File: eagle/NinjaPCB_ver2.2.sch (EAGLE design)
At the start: 70 parts, among them IC1 ANALOGSW_AD_SOT23-6, IC2 NAU7802, Q1 IRLB3813PBF, Q2 CJ2302, Q3 CJ2302, Q4 S9013, Q5 S9013, Q6 S9013

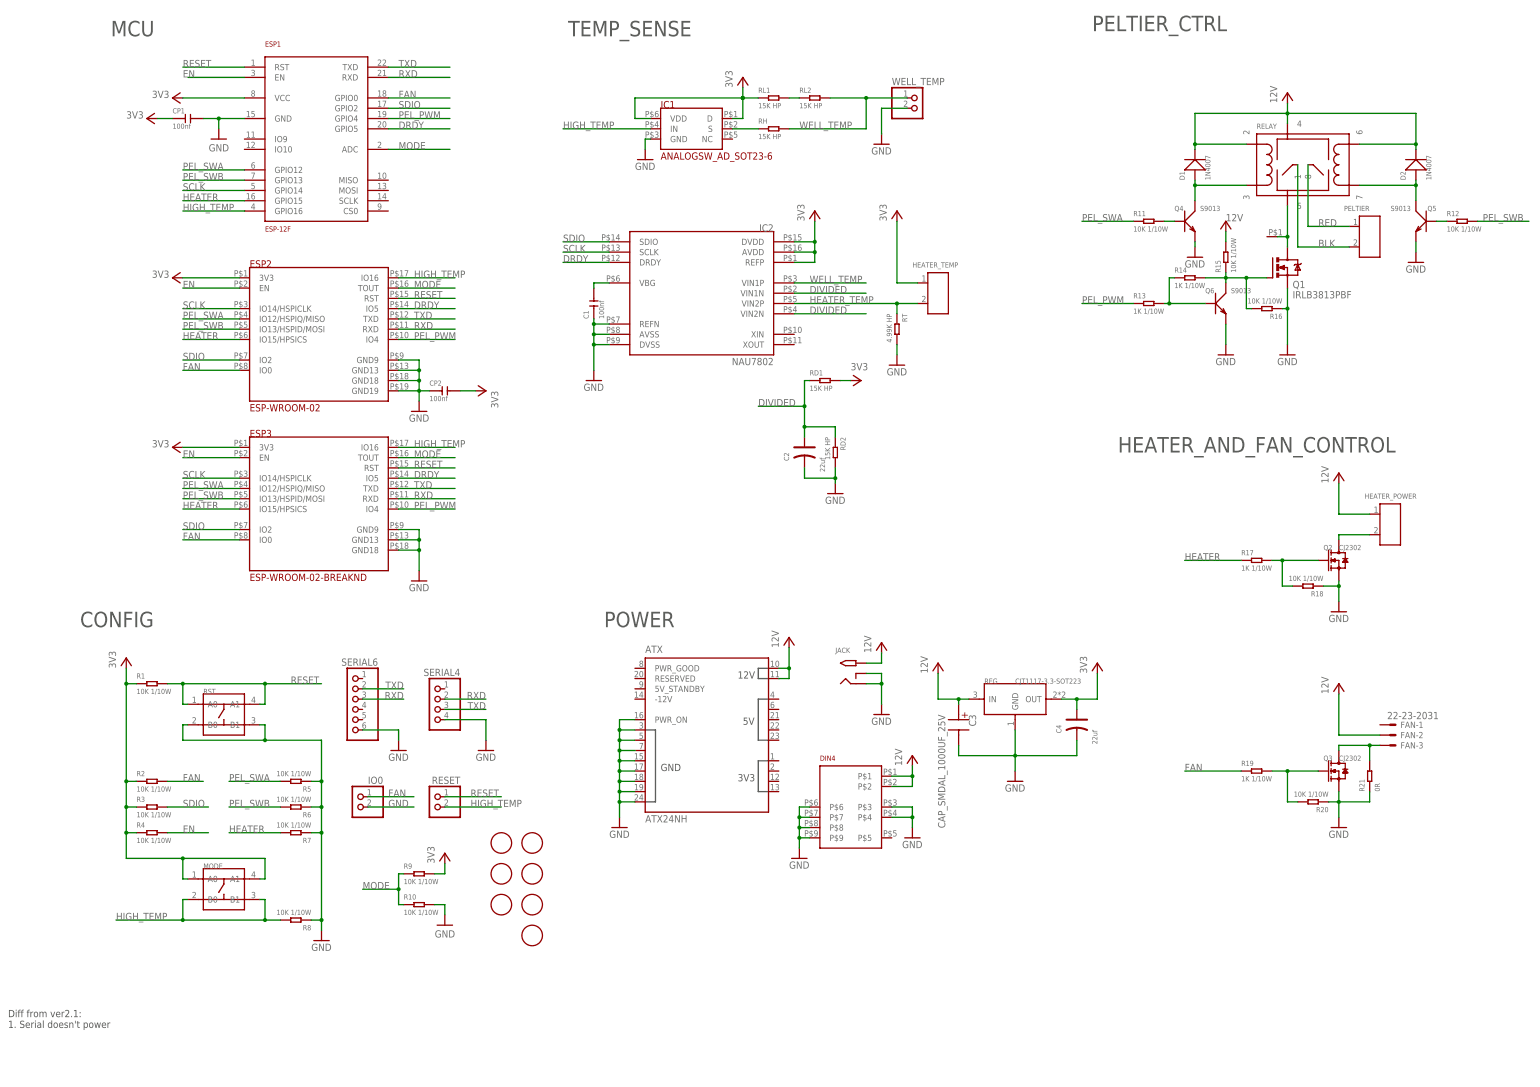
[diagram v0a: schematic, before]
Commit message: sync
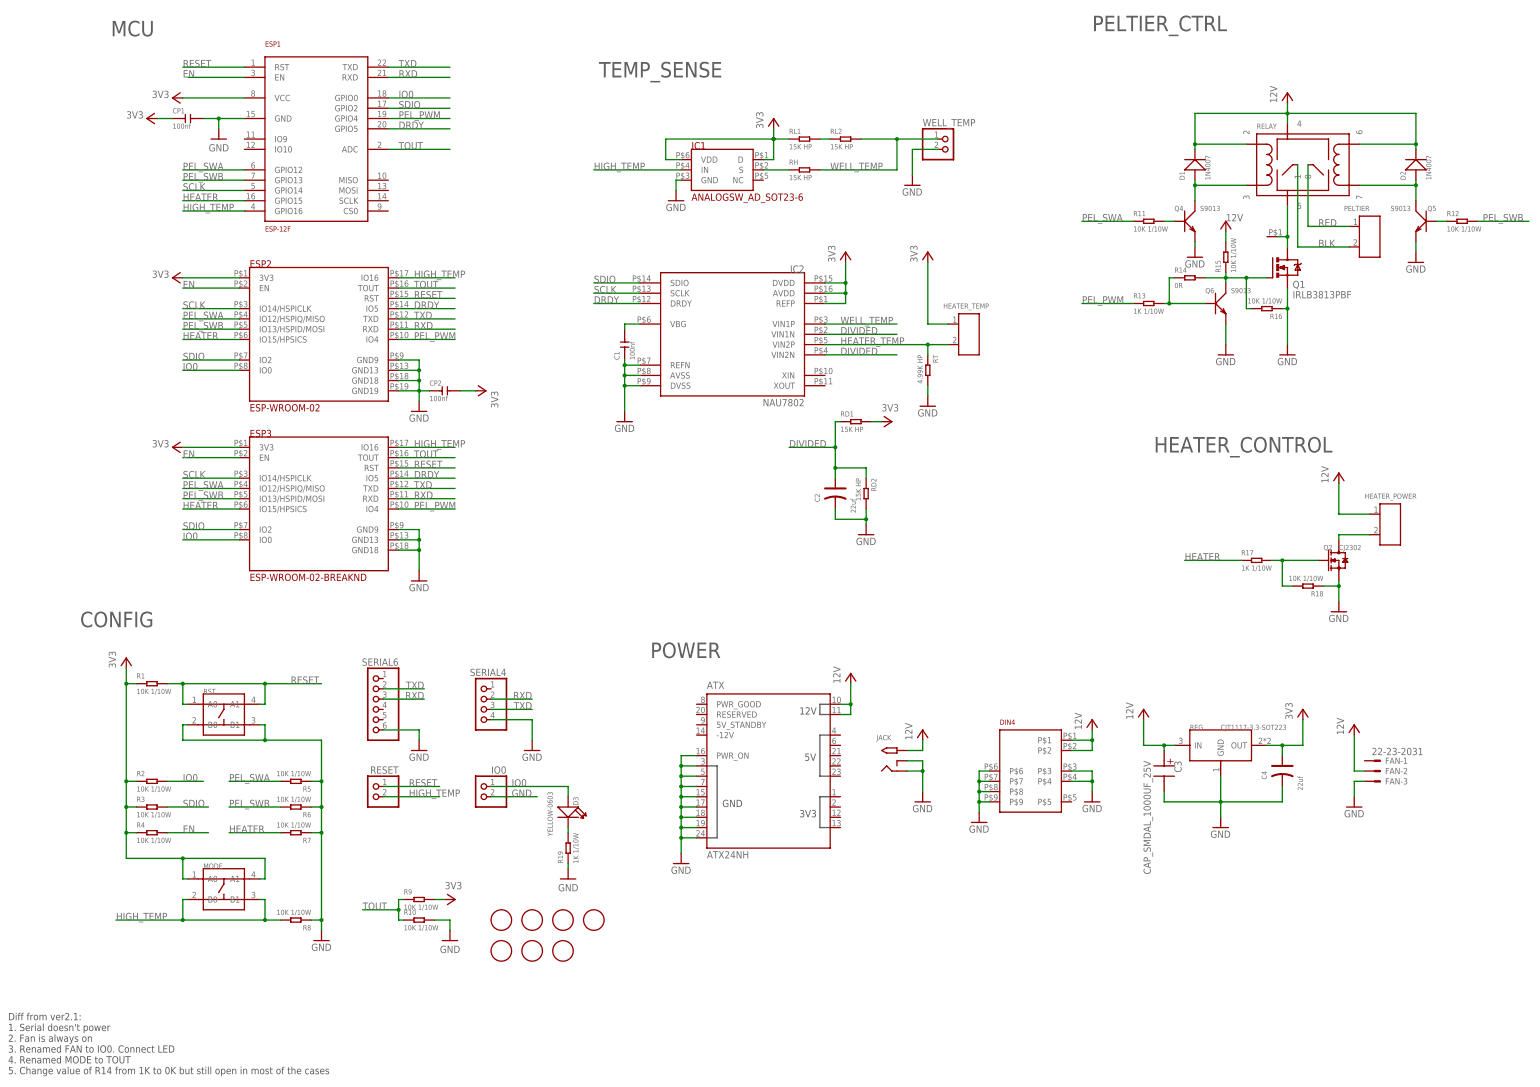
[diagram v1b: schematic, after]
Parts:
- removed Q3: CJ2302, Seeed-Transistor:SMD-MOSFET-N-CH-20V-2.1A-CJ2302(SOT-23)
- removed R20: 10K 1/10W, Seeed-Resistor:SMD-RES-10K-5%-1/10W(0603)
- removed R21: 0R, Seeed-Resistor:SMD-RES-0R-5%-1/10W(0603)
- added D3: YELLOW-0603, Seeed-LED:SMD-LED-CLEAR-YELLOW(0603)
- R14: value 1K 1/10W -> 0R; device Seeed-Resistor:SMD-RES-1K-5%-1/10W(0603) -> Seeed-Resistor:SMD-RES-0R-5%-1/10W(0603)
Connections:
- net MODE renamed TOUT
- removed net FAN: ESP1.GPIO0, ESP2.IO0, ESP3.IO0, IO0.1, R19.1, R2.2
- removed net N$8: Q3.G, R19.2, R20.2
- new net IO0: D3.+, ESP1.GPIO0, ESP2.IO0, ESP3.IO0, IO0.1, R2.2
- net GND: now also FAN-3.S, R19.1; no longer Q3.S, R20.1, R21.1
- net N$4: now also D3.-, R19.2; no longer FAN-3.S, Q3.D, R21.2
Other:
- note added: "Diff from ver2.1: 1. Serial doesn't power 2. Fan is always on 3. Renamed FAN to IO0. Connect LED 4. Renamed MODE to TOUT 5. Change value of R14 from 1K to 0K but still open in most of the cases"
- note added: "HEATER_CONTROL"
- note removed: "Diff from ver2.1: 1. Serial doesn't power"
- note removed: "HEATER_AND_FAN_CONTROL"
- moved on the sheet: ATX, C1, C2, C3, C4, DIN4, FAN-1, FAN-2, FAN-3, HEATER_TEMP, IC1, IC2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
